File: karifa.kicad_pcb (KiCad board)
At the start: 2 copper layers, 38.2 x 54.8 mm, 35 parts, among them J1 Conn_01x04, Q1 AO3401A, Q2 AO3401A, Q3 AO3401A, SW1 SW_DPST_x2, U1 STC8G1K08-SOP16

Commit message: panelizacio
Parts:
- added T1: Tab, kikit:Tab, F.Cu at (130.2, 99.1)
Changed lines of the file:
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@@
     )
+  )
+  (footprint "kikit:Tab" (layer "F.Cu")
+    (at 130.175 99.08 90)
+    (descr "A symbol representing annotation for tab placement")
+    (property "Sheetfile" "karifa.kicad_sch")
+    (property "Sheetname" "")
+    (property "exclude_from_bom" "")
+    (attr exclude_from_pos_files exclude_from_bom)
+    (fp_text reference "T1" (at 0 -2 90) (layer "F.SilkS") hide
+      (effects (font (size 1 1) (thickness 0.15)))
+    )
+    (fp_text value "Tab" (at -2.75 -1 90) (layer "Dwgs.User")
+      (effects (font (size 1.2 1.2) (thickness 0.2)))
+    )
+    (fp_text user "KIKIT: width: 3mm" (at -5.5 0) (layer "Dwgs.User")
+      (effects (font (size 1 1) (thickness 0.15)))
+    )
+    (fp_line (start 0.25 0) (end -2.75 0) (layer "Dwgs.User") (width 0.3))
+    (fp_line (start 0.25 1) (end 0.25 -1) (layer "Dwgs.User") (width 0.3))
+    (fp_line (start 0.25 0) (end -0.75 -1) (layer "Dwgs.User") (width 0.3))
+    (fp_line (start 0.25 0) (end -0.75 1) (layer "Dwgs.User") (width 0.3))
   )
   (footprint "Connector_PinHeader_1.27mm:PinHeader_1x04_P1.27mm_Vertical" (layer "F.Cu")

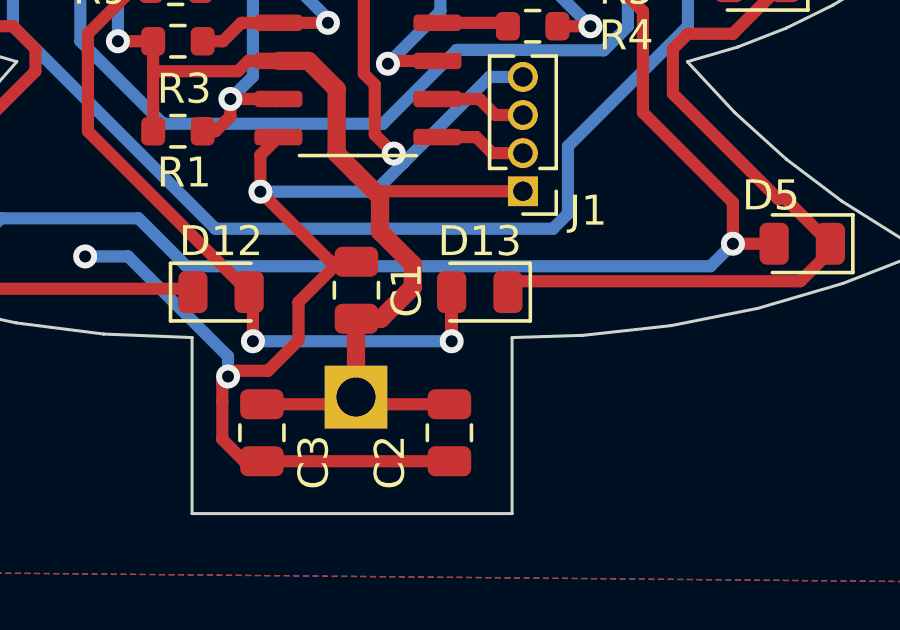
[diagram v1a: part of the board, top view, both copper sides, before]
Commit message: kisebb javitasok
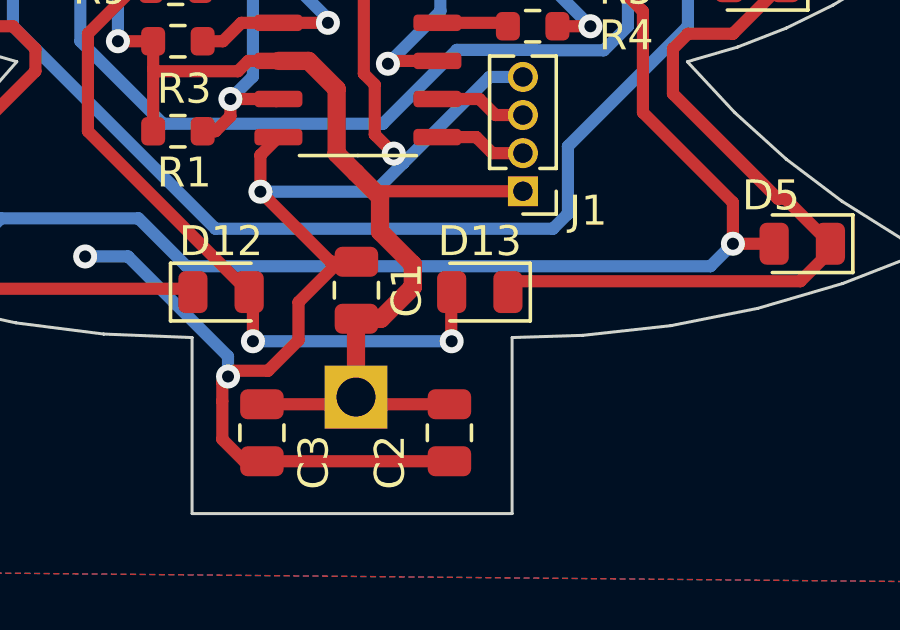
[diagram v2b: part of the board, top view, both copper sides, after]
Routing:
- net Net-(D12-Pad2): track 25.3 -> 23.5 mm
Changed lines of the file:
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@@
   (segment (start 126.75 93.25) (end 126.75 91.736) (width 0.4064) (layer "F.Cu") (net 10))
   (segment (start 126.625 91.611) (end 126.611 91.611) (width 0.4064) (layer "F.Cu") (net 10))
-  (segment (start 133.264 91.5) (end 133.375 91.611) (width 0.4064) (layer "F.Cu") (net 10))
   (segment (start 126.75 91.736) (end 126.625 91.611) (width 0.4064) (layer "F.Cu") (net 10))
   (segment (start 133.361 93.236) (end 133.361 91.611) (width 0.4064) (layer "F.Cu") (net 10))
   (segment (start 122.75 81.5) (end 123.35 81.5) (width 0.4064) (layer "F.Cu") (net 10))
-  (segment (start 133.375 91.611) (end 133.375 93.25) (width 0.4064) (layer "F.Cu") (net 10))
   (segment (start 121.25 83) (end 122.75 81.5) (width 0.4064) (layer "F.Cu") (net 10))
   (segment (start 121.25 86.25) (end 121.25 83) (width 0.4064) (layer "F.Cu") (net 10))

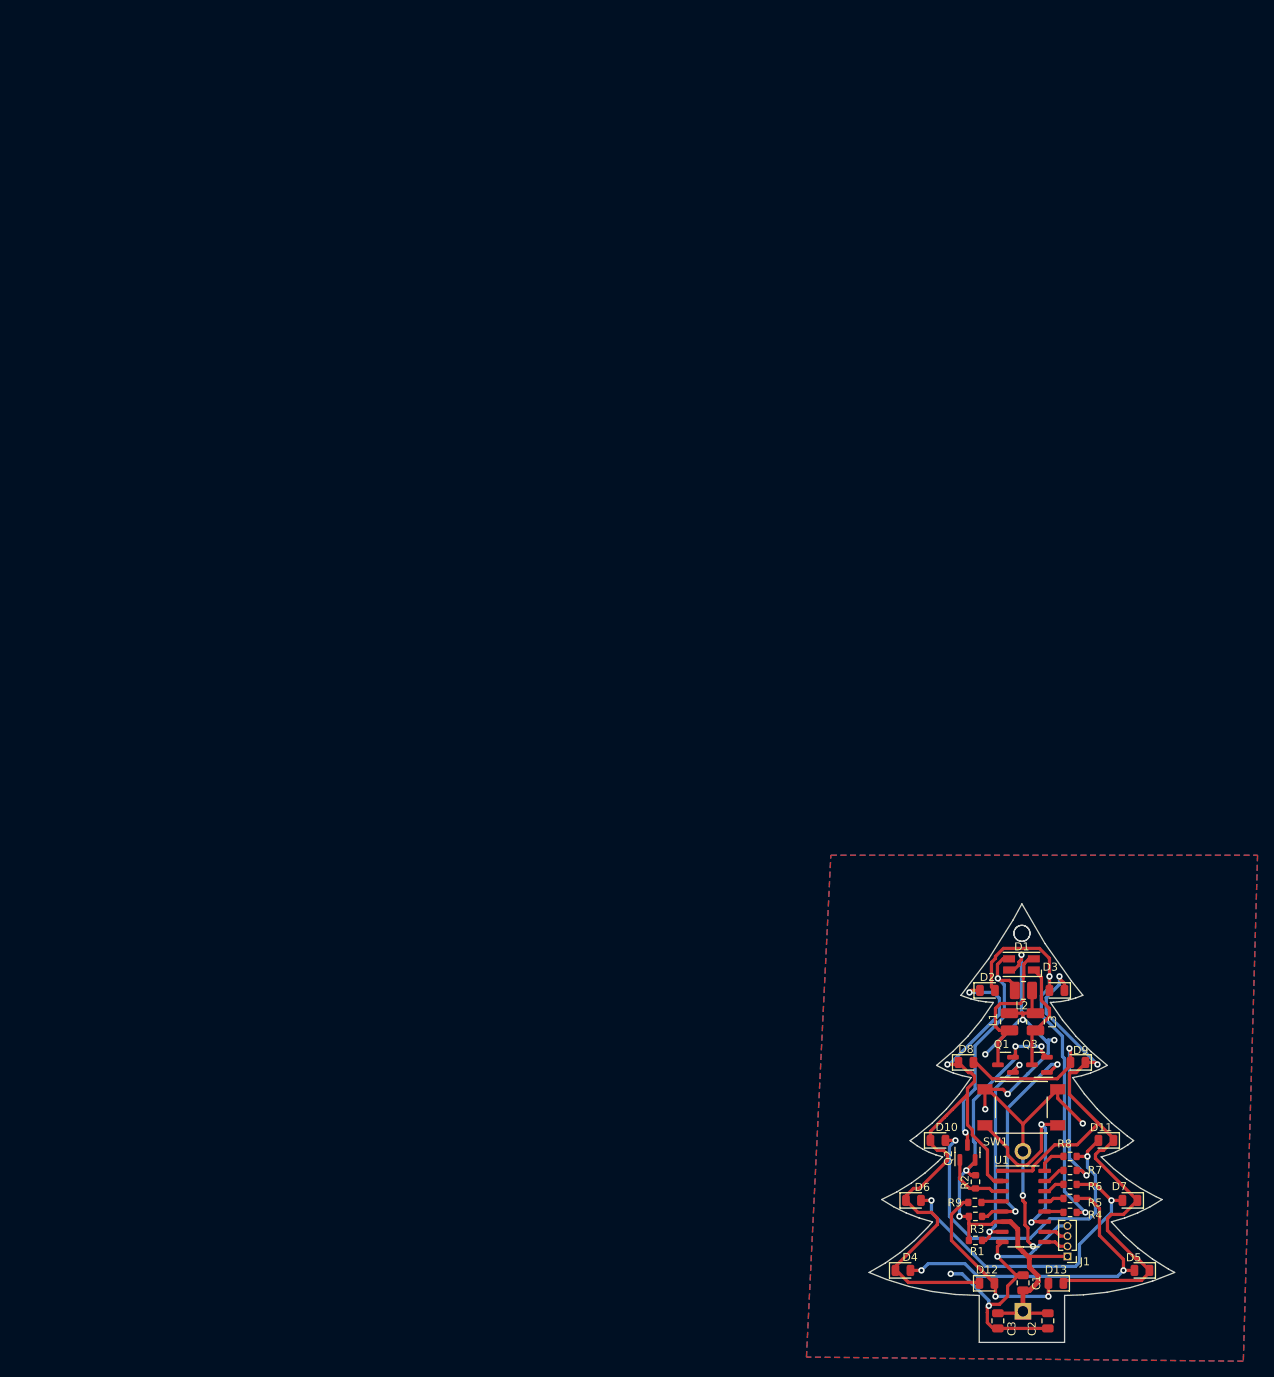
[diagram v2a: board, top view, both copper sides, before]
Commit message: hullocsillag
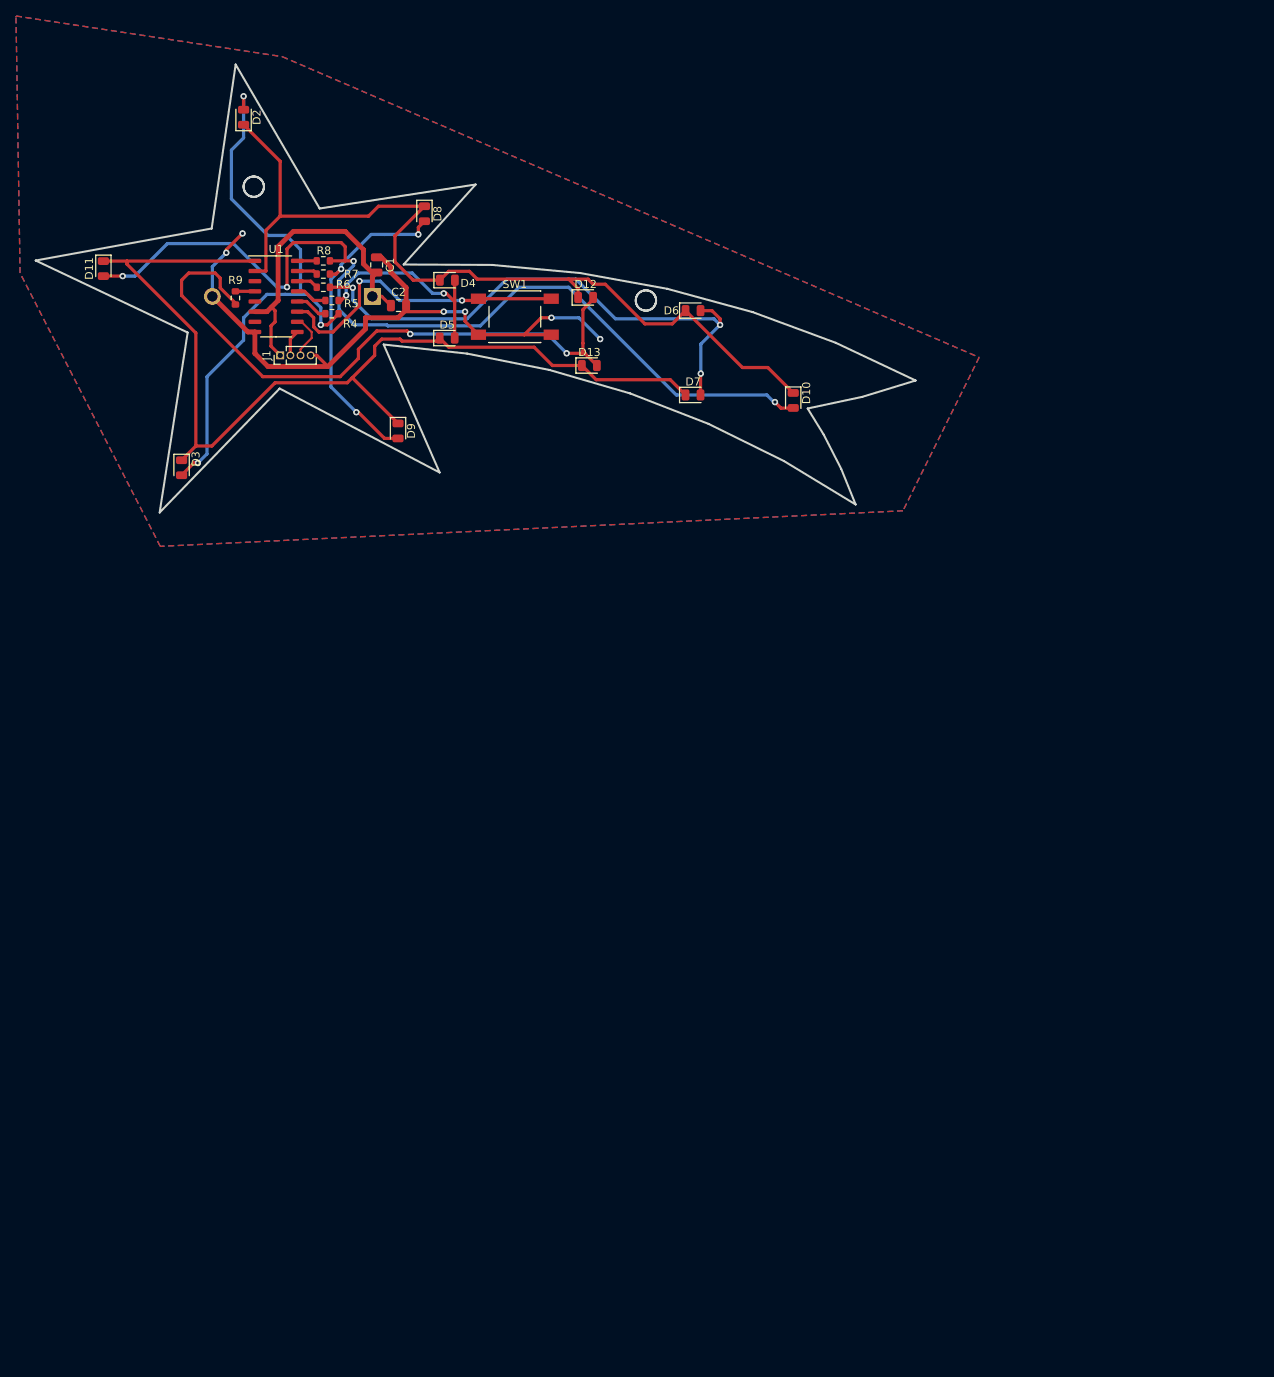
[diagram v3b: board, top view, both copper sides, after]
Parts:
- removed C3: 10uF, Capacitor_SMD:C_0805_2012Metric
- removed D1: LED_ARGB, LED_SMD:LED_RGB_Wuerth-PLCC4_3.2x2.8mm_150141M173100
- removed L1, L2, L3: L, Inductor_SMD:L_1008_2520Metric
- removed Q1, Q2, Q3: AO3401A, Package_TO_SOT_SMD:SOT-23
- removed R1, R2, R3: 100k, Resistor_SMD:R_0603_1608Metric
- removed T1: Tab, kikit:Tab
- BT1: footprint karifa:CR2032_Holder -> valami:CR2032_Holder
- SW1: footprint karifa:SW_Push_K2-1102SP -> valami:SW_Push_K2-1102SP
- moved D11 166.1 mm to (15.2, -35.2), turned to -90 degrees
- moved C1 150.7 mm to (49.4, -35.7)
- moved BT1 150.7 mm to (48.9, -31.8), turned to 180 degrees
- moved C2 150.6 mm to (52.1, -30.6), turned to 0 degrees
- moved J1 149.6 mm to (37.3, -24.4), turned to 90 degrees
- moved U1 147.2 mm to (36.8, -31.8)
- moved R9 146.0 mm to (31.8, -31.6), turned to 90 degrees
- moved R6 145.9 mm to (42.7, -32.9)
- moved R7 145.8 mm to (42.7, -34.5)
- moved R8 145.8 mm to (42.7, -36.2)
- moved R4 145.4 mm to (43.8, -29.6)
- moved D5 145.3 mm to (58.2, -26.5), turned to 0 degrees
- moved R5 145.3 mm to (43.8, -31.2)
- moved D2 143.4 mm to (32.8, -54.2), turned to 90 degrees
- moved D4 136.3 mm to (58.2, -33.8)
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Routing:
- net Net-(D10-Pad2): track 43.1 -> 116.9 mm, vias 2 -> 4
- net Net-(D12-Pad2): track 23.5 -> 80.1 mm
- net /MPX1: track 81.9 -> 126.9 mm, vias 2 -> 0
- net GND: track 119.0 -> 86.6 mm, vias 12 -> 6
- net Net-(D1-Pad2): track 30.3 -> 0.00 mm, vias 2 -> 0
- net VCC: track 69.6 -> 39.7 mm, vias 4 -> 0
- net /MPX2: track 81.5 -> 111.0 mm, vias 2 -> 0
- net Net-(D6-Pad2): track 40.3 -> 69.1 mm, vias 2 -> 3
- net /P5.4: track 28.0 -> 0.00 mm, vias 2 -> 0
- net /P5.5: track 27.0 -> 0.00 mm, vias 2 -> 0
- net Net-(D2-Pad2): track 49.6 -> 71.7 mm, vias 2 -> 3
- net Net-(D1-Pad4): track 19.4 -> 0.00 mm
- net Net-(D4-Pad2): track 41.7 -> 25.4 mm
- net Net-(D1-Pad3): track 13.6 -> 0.00 mm
- net Net-(SW1-Pad1): track 30.6 -> 39.0 mm
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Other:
- board size 38.2 x 54.8 mm -> 110 x 56 mm
